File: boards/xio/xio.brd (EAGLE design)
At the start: 170 x 170 mm, 241 parts, among them CN3 J00-0065NL, U2 LAN8742A-CZ, X2 USB-A, Y1 NX3225SA-12.000MHZ-STD-CSR-1, Y2 NX3225SA-12.000MHZ-STD-CSR-1, Y3 NX3225SA-25.000MHZ-STD-CSR-1

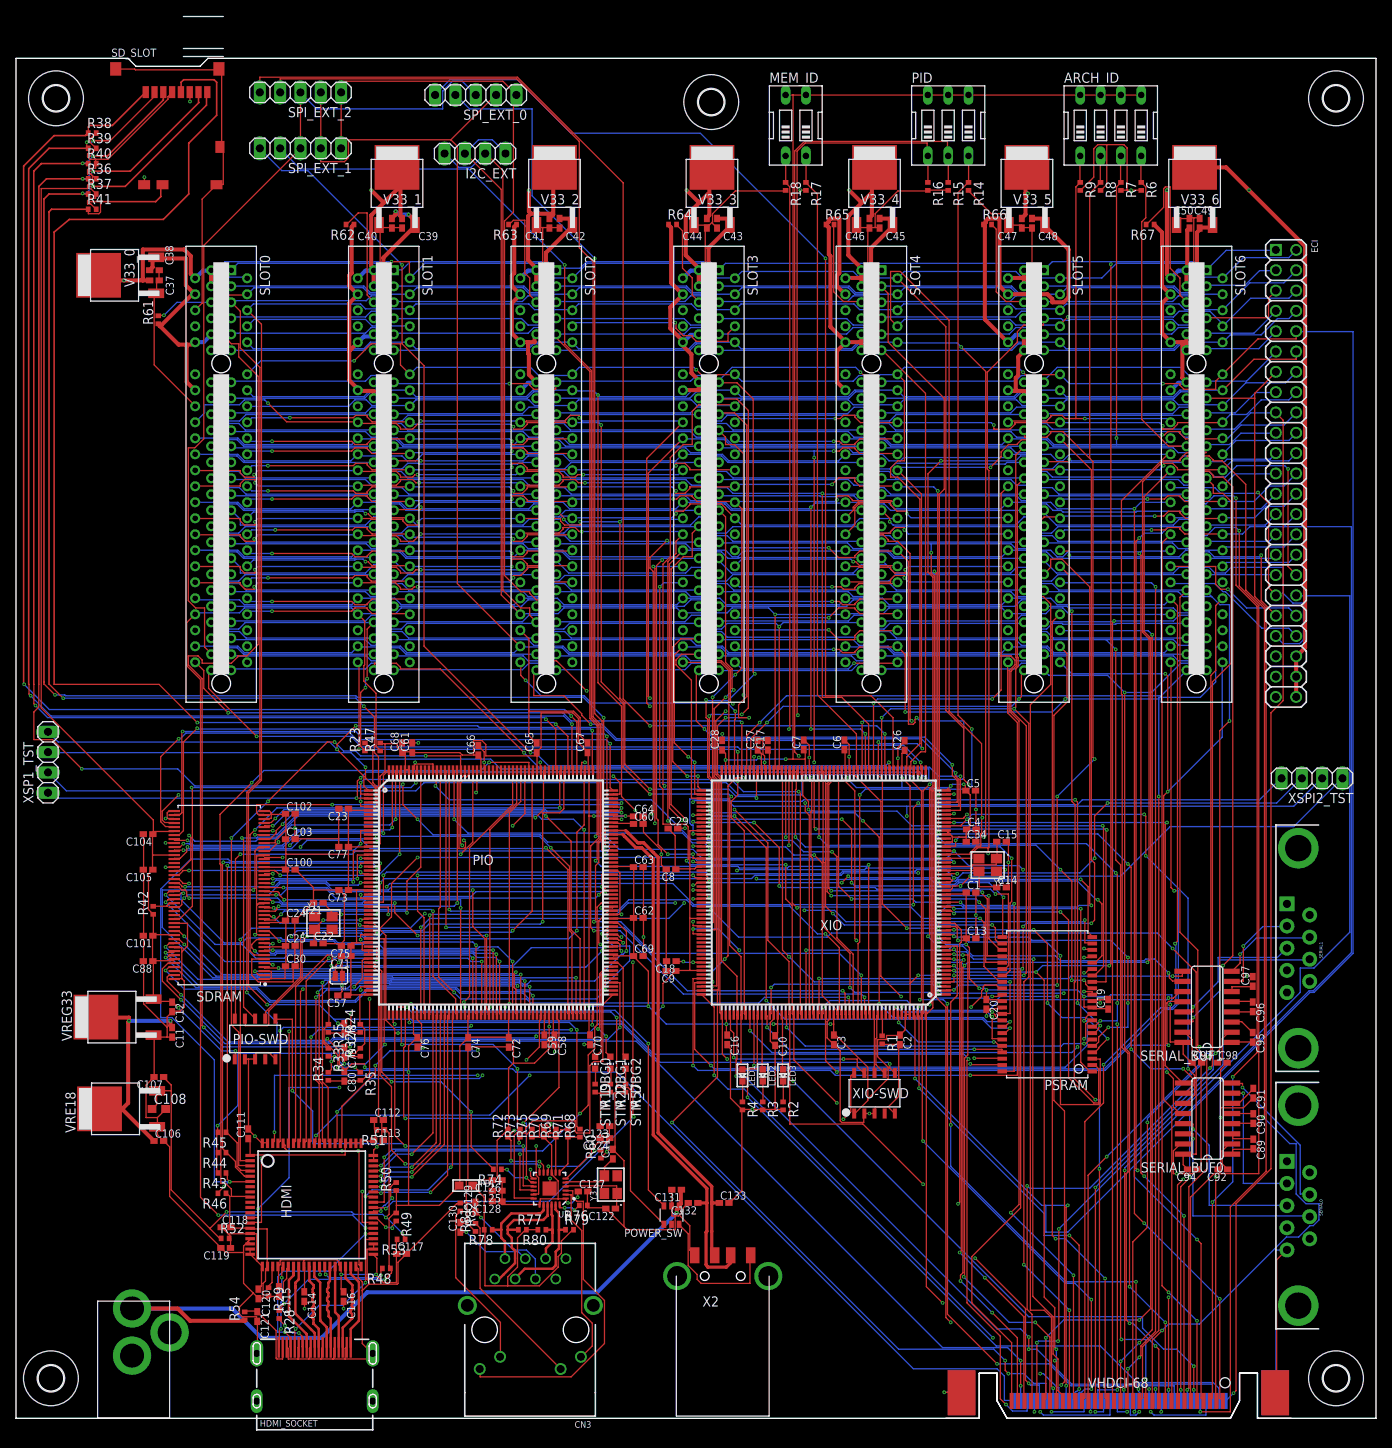
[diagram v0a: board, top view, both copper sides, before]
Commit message: Revision ready for routing for DR
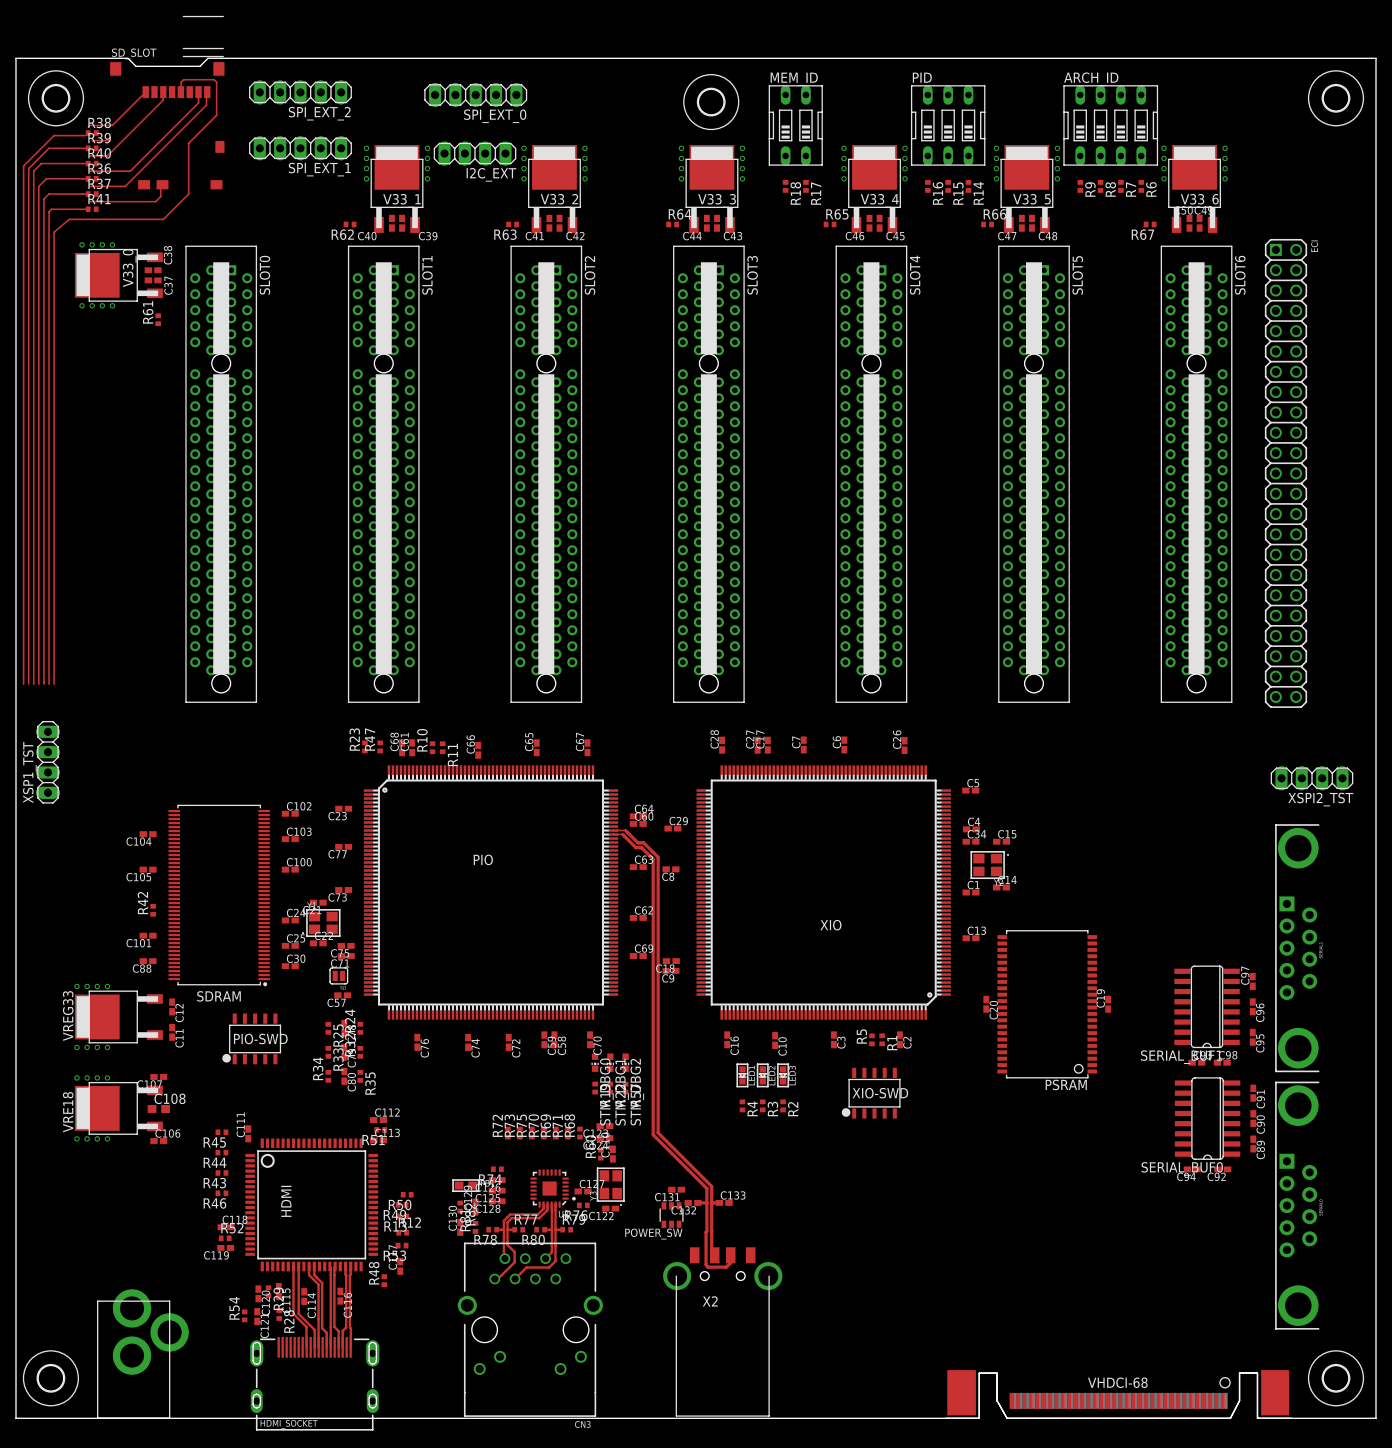
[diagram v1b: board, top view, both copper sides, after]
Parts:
- added R10, R11, R5: 0R, rcl:R0402
- added R12, R13: 2.7k, rcl:R0402
- R2, R3, R4: value 330 -> 1K
- V33_0, V33_1, V33_2, V33_3, V33_4, V33_5, V33_6, VREG33: value AP7363-330-13 -> AP7363-33D-13
- moved R50 1.72 mm to (48.9, 27.9), turned to 180 degrees
- moved R49 1.68 mm to (48.3, 26.7), turned to 180 degrees
- moved C117 1.56 mm to (48.0, 19.0), turned to 90 degrees
- moved R48 1.55 mm to (46.0, 17.2), turned to 90 degrees
- moved R53 0.79 mm to (48.3, 21.6)
- moved R78 0.56 mm to (59.6, 23.6)
- moved R77 0.46 mm to (62.8, 23.6)
- moved C116 0.41 mm to (40.5, 15.3)
- moved R79 0.36 mm to (68.8, 23.6)
- moved VRE18 0.29 mm to (10.2, 38.7)
- moved VREG33 0.17 mm to (10.2, 50.2)
- moved C37 0.16 mm to (17.1, 142.2)
- moved C38 0.16 mm to (17.1, 143.5)
- moved V33_0 0.16 mm to (10.2, 142.9)
- moved R80 0.15 mm to (65.6, 23.6)
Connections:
- new net N$6: PIO.197, R10.1, R11.2
- net +3V3: now also R11.1, R5.1
- net +5V: now also R12.1, R13.1
- net DDSCL: now also R12.2
- net DDSDA: now also R13.2
- net GND: now also R10.2, SLOT0.B9, SLOT1.B15, SLOT2.B13, SLOT2.B9, SLOT3.B13, SLOT3.B15, SLOT4.B9, SLOT6.B11, SLOT6.B13, SLOT6.B9; no longer PIO.197, SLOT2.B12, SLOT3.B12, SLOT4.B15, SLOT6.B12, SLOT6.B15
- net N$11: now also R5.2
- net S1_V33: no longer SLOT0.B9
- net S2_V33: no longer SLOT1.B15
- net S3_V33: now also SLOT2.B12; no longer SLOT2.B13, SLOT2.B9
- net S4_V33: now also SLOT3.B12; no longer SLOT3.B13
- net S5_V33: now also SLOT4.B15; no longer SLOT4.B9
- net S7_V33: now also SLOT6.B12, SLOT6.B15; no longer SLOT6.B11, SLOT6.B13, SLOT6.B9
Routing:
- net +3V3: track 1015.9 -> 0.00 mm, vias 34 -> 0
- net GND: track 918.4 -> 0.00 mm, vias 62 -> 0
- net +5V: track 369.2 -> 0.00 mm, vias 11 -> 72
- net VHDCI_AUDIO_SIO: track 368.0 -> 0.00 mm, vias 4 -> 0
- net VHDCI_AUDIO_L: track 358.2 -> 0.00 mm, vias 4 -> 0
- net VHDCI_A5: track 348.3 -> 0.00 mm, vias 6 -> 0
- net VHDCI_A8: track 346.2 -> 0.00 mm, vias 3 -> 0
- net VHDCI_A12: track 339.8 -> 0.00 mm, vias 3 -> 0
- net VHDCI_AUDIO_R: track 337.2 -> 0.00 mm, vias 3 -> 0
- net VHDCI_A6: track 336.2 -> 0.00 mm, vias 7 -> 0
- net VHDCI_A2: track 334.2 -> 0.00 mm, vias 4 -> 0
- net I2C_SCL: track 328.1 -> 0.00 mm, vias 3 -> 0
- net VHDCI_D2: track 325.5 -> 0.00 mm, vias 6 -> 0
- net I2C_SDA: track 324.2 -> 0.00 mm, vias 4 -> 0
- net VHDCI_A1: track 320.9 -> 0.00 mm, vias 4 -> 0
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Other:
- board text added: "1mm max len diff"
- board text added: "TX:4mm RX: 6mm"
- board text removed: "Add vias to +3v3 around vRegs XIO:BOOT0 ought to have no-stuff pull-up Label for XIO:XSPI XIO:LED ought to be 1k ? XIO:PSRAM - check pins XIO:Serial IO - move gnd/power pins PIO:BOOT0 needs pullup/down Labels for SD-Card and ADC sections Notes on SDRAM lengths Label for Audio/video section into HDMI Move PIO:Video-in to 14/19"

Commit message: Checkpoint
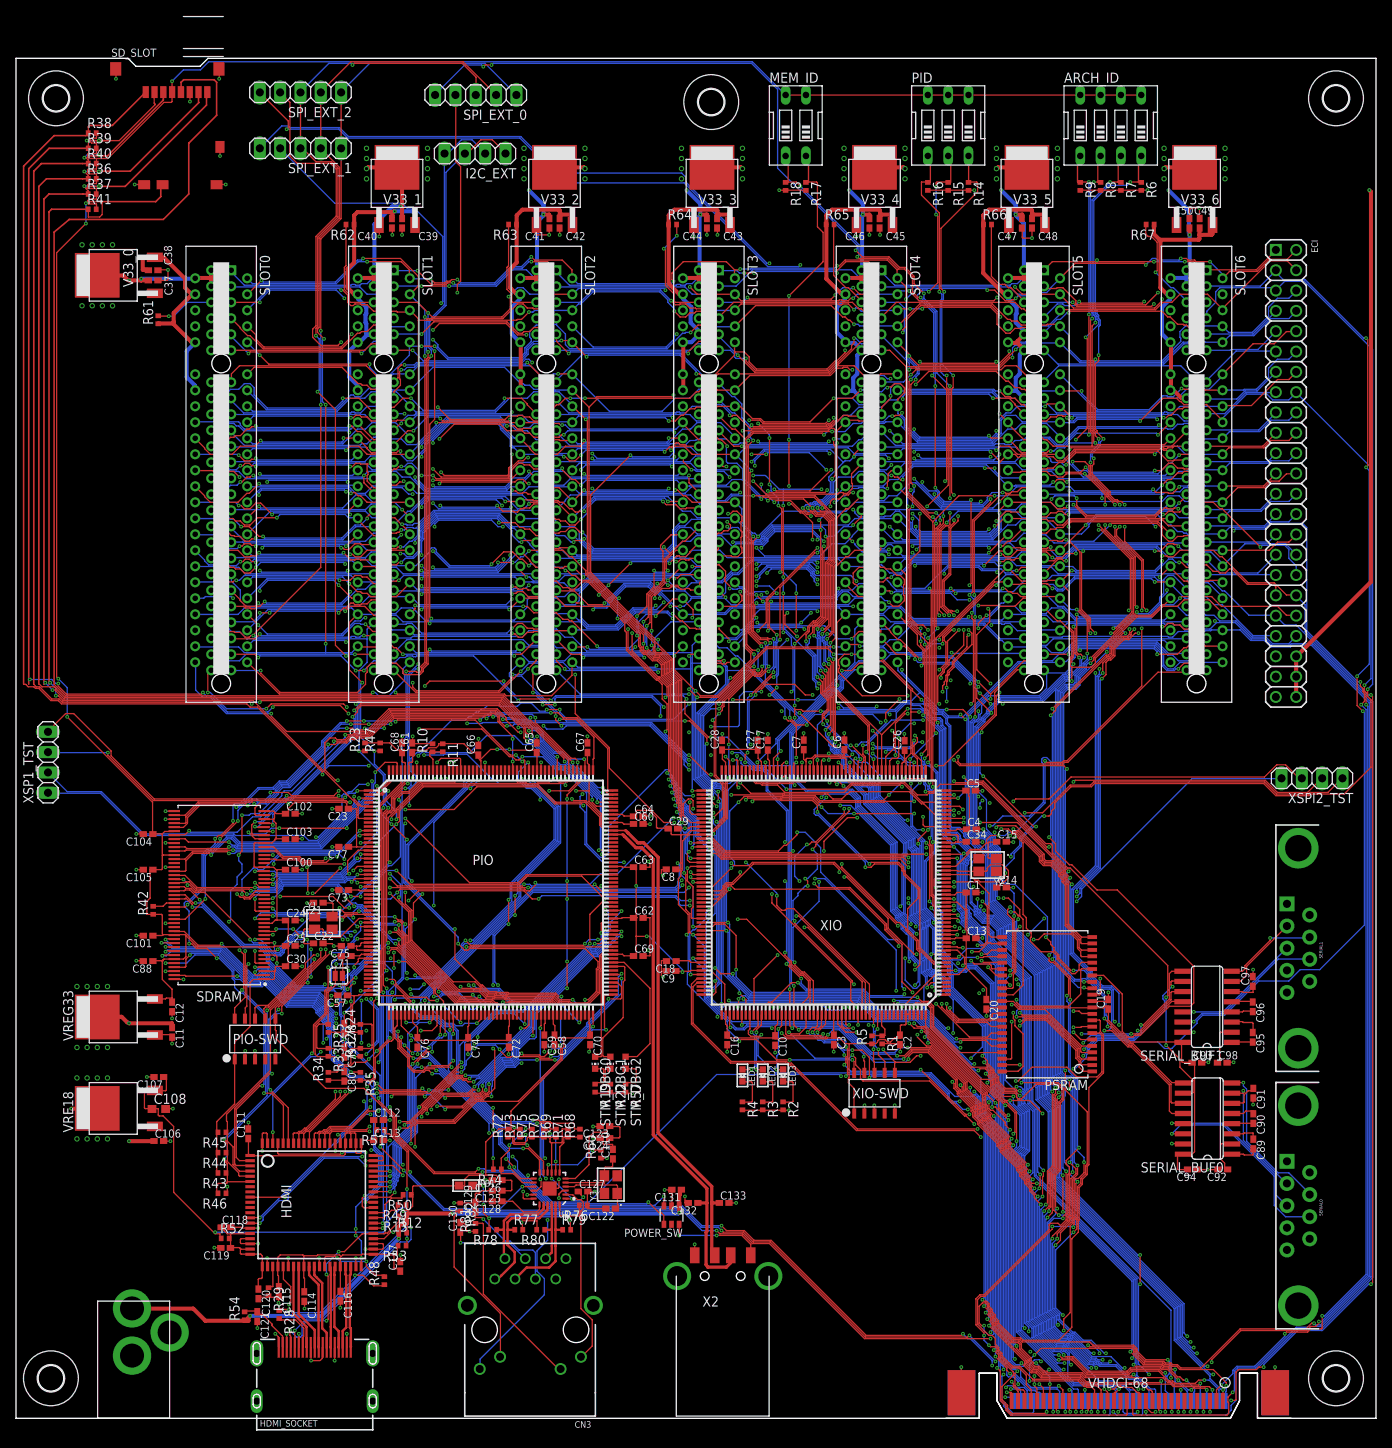
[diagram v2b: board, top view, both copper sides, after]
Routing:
- net +3V3: track 0.00 -> 933.1 mm, vias 0 -> 22
- net VHDCI_A11: track 0.00 -> 383.4 mm, vias 0 -> 15
- net VHDCI_A0: track 0.00 -> 368.1 mm, vias 0 -> 10
- net VHDCI_AUDIO_SIO: track 0.00 -> 360.9 mm, vias 0 -> 17
- net !VHDCI_MPD!: track 0.00 -> 356.5 mm, vias 0 -> 12
- net VHDCI_AUDIO_R: track 0.00 -> 349.3 mm, vias 0 -> 24
- net VHDCI_AUDIO_L: track 0.00 -> 344.3 mm, vias 0 -> 23
- net VHDCI_A9: track 0.00 -> 332.5 mm, vias 0 -> 17
- net VHDCI_D1: track 0.00 -> 332.4 mm, vias 0 -> 21
- net VHDCI_A6: track 0.00 -> 330.8 mm, vias 0 -> 14
- net VHDCI_A8: track 0.00 -> 329.5 mm, vias 0 -> 11
- net VHDCI_REF: track 0.00 -> 328.4 mm, vias 0 -> 16
- net VHDCI_RST: track 0.00 -> 325.5 mm, vias 0 -> 12
- net VHDCI_A12: track 0.00 -> 324.4 mm, vias 0 -> 10
- net VHDCI_A10: track 0.00 -> 323.2 mm, vias 0 -> 14
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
